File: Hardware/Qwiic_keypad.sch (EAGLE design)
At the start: 26 parts, among them J3 PTH, J6 AVR_SPI_PROG_3X2TESTPOINTS, U3 ATTINY84

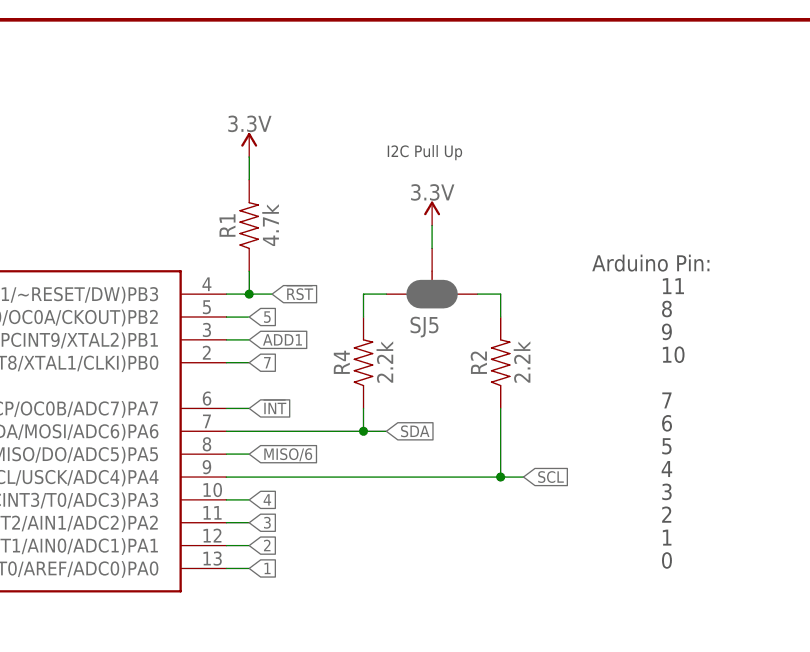
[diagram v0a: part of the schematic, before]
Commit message: Board Revision
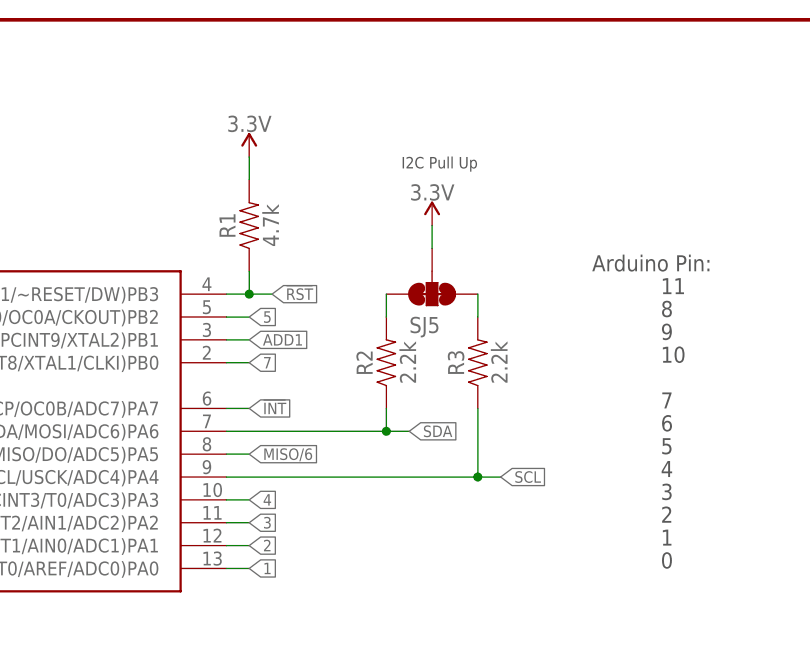
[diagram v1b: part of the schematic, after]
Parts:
- removed R4: 2.2k, SparkFun-Resistors:2.2KOHM-0603-1/10W-1%
- added R3: 2.2k, SparkFun-Resistors:2.2KOHM-0603-1/10W-1%
- SJ5: value JUMPER-SMT_3_2-NC_PASTE_SILK -> JUMPER-SMT_3_2-NC_TRACE_SILK; device SparkFun-Jumpers:JUMPER-SMT_3_2-NC_PASTE_SILK -> SparkFun-Jumpers:JUMPER-SMT_3_2-NC_TRACE_SILK
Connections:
- removed net SCL_PU1: R2.2, SJ5.1
- removed net SDA_PU1: R4.2, SJ5.3
- new net N$2: R2.2, SJ5.3
- new net N$3: R3.2, SJ5.1
- net SCL: now also R3.1; no longer R2.1
- net SDA: now also R2.1; no longer R4.1
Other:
- moved on the sheet: R2
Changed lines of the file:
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@@
 <?xml version="1.0" encoding="utf-8"?>
 <!DOCTYPE eagle SYSTEM "eagle.dtd">
-<eagle version="7.7.0">
+<eagle version="9.0.1">
 <drawing>
 <settings>
 <setting alwaysvectorfont="yes"/>
+<setting keepoldvectorfont="yes"/>
 <setting verticaltext="up"/>
 </settings>
@@
 <part name="LOGO1" library="SparkFun-Aesthetics" deviceset="OSHW-LOGO" device="MINI"/>
 <part name="U$1" library="SparkX" deviceset="SPARKX-LOGO" device="3" value="SPARKX-LOGO3"/>
-<part name="R2" library="SparkFun-Resistors" deviceset="2.2KOHM" device="-0603-1/10W-1%" value="2.2k"/>
-<part name="R4" library="SparkFun-Resistors" deviceset="2.2KOHM" device="-0603-1/10W-1%" value="2.2k"/>
-<part name="SJ5" library="SparkFun-Jumpers" deviceset="JUMPER-SMT_3_2-NC_PASTE" device="_SILK" value=""/>
-<part name="SUPPLY1" library="SparkFun-PowerSymbols" deviceset="3.3V" device=""/>
+<part name="SJ5" library="SparkFun-Jumpers" deviceset="JUMPER-SMT_3_2-NC_TRACE" device="_SILK" value=""/>
 <part name="J1" library="SparkFun-Connectors" deviceset="CONN_01" device="PTH_NO_SILK_YES_STOP"/>
 <part name="GND2" library="SparkFun" deviceset="GND" device=""/>
@@
 <part name="H2" library="SparkFun-Hardware" deviceset="STAND-OFF" device=""/>
 <part name="J8" library="SparkFun-Connectors" deviceset="CONN_07" device="NO_SILK"/>
+<part name="R2" library="SparkFun-Resistors" deviceset="2.2KOHM" device="-0603-1/10W-1%" value="2.2k"/>
+<part name="R3" library="SparkFun-Resistors" deviceset="2.2KOHM" device="-0603-1/10W-1%" value="2.2k"/>
+<part name="SUPPLY1" library="SparkFun-PowerSymbols" deviceset="3.3V" device=""/>
 </parts>
 <sheets>
@@
 <text x="128.778" y="77.724" size="1.778" layer="97">Power
 Indicator</text>
-<text x="101.6" y="170.18" size="1.27" layer="97">I2C Pull Up</text>
+<text x="111.76" y="170.18" size="1.27" layer="97" rot="R180">I2C Pull Up</text>
 <wire x1="172.72" y1="185.42" x2="172.72" y2="91.44" width="0.2032" layer="97"/>
 <text x="124.46" y="157.48" size="1.778" layer="97" ratio="15">Arduino Pin:</text>
@@
 <instance part="LOGO1" gate="G$1" x="121.92" y="22.86"/>
 <instance part="U$1" gate="G$1" x="121.92" y="7.62"/>
-<instance part="R2" gate="G$1" x="114.3" y="147.32" rot="R90"/>
-<instance part="R4" gate="G$1" x="99.06" y="147.32" rot="R90"/>
 <instance part="SJ5" gate="G$1" x="106.68" y="154.94" smashed="yes" rot="R270">
 <attribute name="NAME" x="104.14" y="150.622" size="1.778" layer="95" font="vector"/>
 <attribute name="VALUE" x="106.299" y="152.4" size="1.778" layer="96" font="vector" rot="R270" align="top-left"/>
 </instance>
-<instance part="SUPPLY1" gate="G$1" x="106.68" y="162.56"/>
 <instance part="J1" gate="G$1" x="53.34" y="10.16"/>
 <instance part="GND2" gate="1" x="203.2" y="45.72" rot="MR0"/>
@@
 <instance part="H2" gate="G$1" x="236.22" y="30.48"/>
 <instance part="J8" gate="G$1" x="20.32" y="25.4"/>
+<instance part="R2" gate="G$1" x="101.6" y="147.32" rot="R90"/>
+<instance part="R3" gate="G$1" x="111.76" y="147.32" rot="R90"/>
+<instance part="SUPPLY1" gate="G$1" x="106.68" y="162.56"/>
 </instances>
 <busses>
@@
 </segment>
 <segment>
-<wire x1="106.68" y1="160.02" x2="106.68" y2="162.56" width="0.1524" layer="91"/>
-<pinref part="SUPPLY1" gate="G$1" pin="3.3V"/>
-<pinref part="SJ5" gate="G$1" pin="2"/>
-</segment>
-<segment>
 <pinref part="U3" gate="G$1" pin="VCC"/>
 <wire x1="33.02" y1="154.94" x2="30.48" y2="154.94" width="0.1524" layer="91"/>
@@
 <wire x1="134.62" y1="71.12" x2="134.62" y2="68.58" width="0.1524" layer="91"/>
 </segment>
+<segment>
+<wire x1="106.68" y1="160.02" x2="106.68" y2="162.56" width="0.1524" layer="91"/>
+<pinref part="SUPPLY1" gate="G$1" pin="3.3V"/>
+<pinref part="SJ5" gate="G$1" pin="2"/>
+</segment>
 </net>
 <net name="GND" class="0">
@@
 <wire x1="83.82" y1="142.24" x2="86.36" y2="142.24" width="0.1524" layer="91"/>
 <label x="86.36" y="142.24" size="1.27" layer="95" xref="yes"/>
-</segment>
-</net>
-<net name="SCL_PU1" class="0">
-<segment>
-<pinref part="SJ5" gate="G$1" pin="1"/>
-<pinref part="R2" gate="G$1" pin="2"/>
-<wire x1="111.76" y1="154.94" x2="114.3" y2="154.94" width="0.1524" layer="91"/>
-<wire x1="114.3" y1="154.94" x2="114.3" y2="152.4" width="0.1524" layer="91"/>
-</segment>
-</net>
-<net name="SDA_PU1" class="0">
-<segment>
-<pinref part="SJ5" gate="G$1" pin="3"/>
-<pinref part="R4" gate="G$1" pin="2"/>
-<wire x1="101.6" y1="154.94" x2="99.06" y2="154.94" width="0.1524" layer="91"/>
-<wire x1="99.06" y1="154.94" x2="99.06" y2="152.4" width="0.1524" layer="91"/>
 </segment>
 </net>
@@
 <net name="SCL" class="0">
 <segment>
-<pinref part="U3" gate="G$1" pin="(PCINT4/T1/SCL/USCK/ADC4)PA4"/>
-<wire x1="83.82" y1="134.62" x2="114.3" y2="134.62" width="0.1524" layer="91"/>
-<label x="116.84" y="134.62" size="1.27" layer="95" xref="yes"/>
-<pinref part="R2" gate="G$1" pin="1"/>
-<wire x1="114.3" y1="134.62" x2="116.84" y2="134.62" width="0.1524" layer="91"/>
-<wire x1="114.3" y1="142.24" x2="114.3" y2="134.62" width="0.1524" layer="91"/>
-<junction x="114.3" y="134.62"/>
-</segment>
-<segment>
 <pinref part="J6" gate="G$1" pin="3"/>
 <wire x1="200.66" y1="144.78" x2="198.12" y2="144.78" width="0.1524" layer="91"/>
@@
 <label x="68.58" y="40.64" size="1.27" layer="95" rot="MR180" xref="yes"/>
 </segment>
+<segment>
+<pinref part="U3" gate="G$1" pin="(PCINT4/T1/SCL/USCK/ADC4)PA4"/>
+<wire x1="83.82" y1="134.62" x2="111.76" y2="134.62" width="0.1524" layer="91"/>
+<label x="114.3" y="134.62" size="1.27" layer="95" xref="yes"/>
+<pinref part="R3" gate="G$1" pin="1"/>
+<wire x1="111.76" y1="134.62" x2="114.3" y2="134.62" width="0.1524" layer="91"/>
+<wire x1="111.76" y1="142.24" x2="111.76" y2="134.62" width="0.1524" layer="91"/>
+<junction x="111.76" y="134.62"/>
+</segment>
 </net>
 <net name="SDA" class="0">
-<segment>
-<pinref part="U3" gate="G$1" pin="(PCINT6/OC1A/SDA/MOSI/ADC6)PA6"/>
-<wire x1="83.82" y1="139.7" x2="99.06" y2="139.7" width="0.1524" layer="91"/>
-<label x="101.6" y="139.7" size="1.27" layer="95" xref="yes"/>
-<pinref part="R4" gate="G$1" pin="1"/>
-<wire x1="99.06" y1="139.7" x2="101.6" y2="139.7" width="0.1524" layer="91"/>
-<wire x1="99.06" y1="142.24" x2="99.06" y2="139.7" width="0.1524" layer="91"/>
-<junction x="99.06" y="139.7"/>
-</segment>
 <segment>
 <pinref part="J6" gate="G$1" pin="4"/>
@@
 <label x="68.58" y="38.1" size="1.27" layer="95" rot="MR180" xref="yes"/>
 </segment>
-</net>
+<segment>
+<pinref part="U3" gate="G$1" pin="(PCINT6/OC1A/SDA/MOSI/ADC6)PA6"/>
+<wire x1="83.82" y1="139.7" x2="101.6" y2="139.7" width="0.1524" layer="91"/>
+<label x="104.14" y="139.7" size="1.27" layer="95" xref="yes"/>
+<pinref part="R2" gate="G$1" pin="1"/>
+<wire x1="101.6" y1="139.7" x2="104.14" y2="139.7" width="0.1524" layer="91"/>
+<wire x1="101.6" y1="142.24" x2="101.6" y2="139.7" width="0.1524" layer="91"/>
+<junction x="101.6" y="139.7"/>
+</segment>
+</net>
+<net name="N$2" class="0">
+<segment>
+<pinref part="SJ5" gate="G$1" pin="3"/>
+<pinref part="R2" gate="G$1" pin="2"/>
+<wire x1="101.6" y1="154.94" x2="101.6" y2="152.4" width="0.1524" layer="91"/>
+</segment>
+</net>
+<net name="N$3" class="0">
+<segment>
+<pinref part="SJ5" gate="G$1" pin="1"/>
+<pinref part="R3" gate="G$1" pin="2"/>
+<wire x1="111.76" y1="154.94" x2="111.76" y2="152.4" width="0.1524" layer="91"/>
+</segment>
+</net>
